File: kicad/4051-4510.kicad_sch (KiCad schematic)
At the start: 10 parts, among them U19 CD4051B, U20 4510

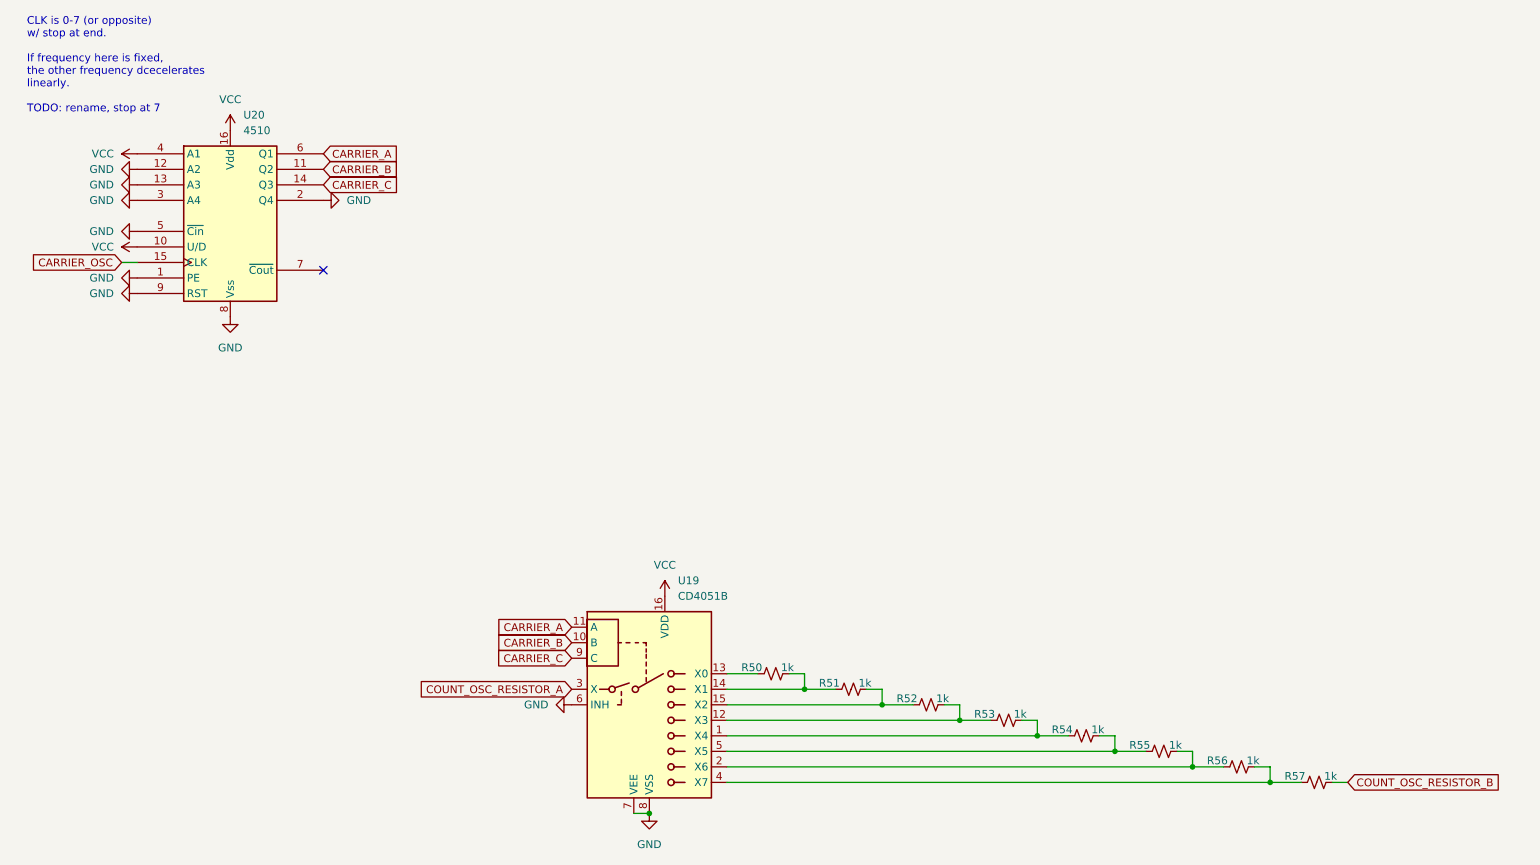
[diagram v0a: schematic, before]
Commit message: CONTINUE
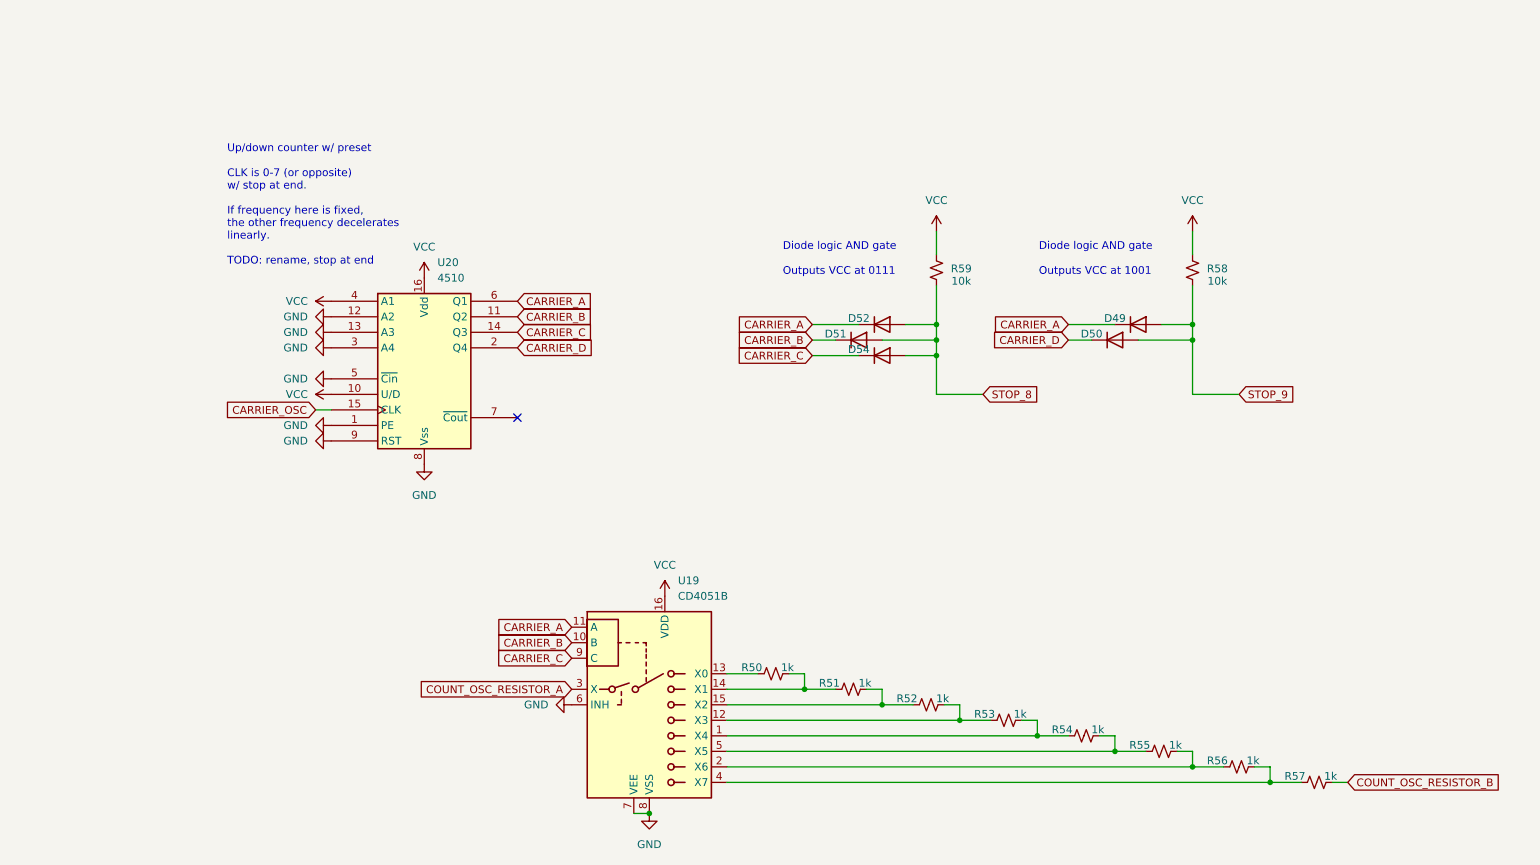
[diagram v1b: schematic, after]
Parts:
- added D49, D50, D51, D52, D54: 1N4148WT, Diode_SMD:D_SOD-523, symbol Diode:1N4148WT
- added R58, R59: 10k, symbol Device:R_Small_US
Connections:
- net CARRIER_A: now also D49.1 (K), D52.1 (K)
- net CARRIER_B: now also D51.1 (K)
- net CARRIER_C: now also D54.1 (K)
- net GND: no longer U20.2 (Q4)
- net VCC: now also R58.2, R59.2
- new net CARRIER_D: D50.1 (K), U20.2 (Q4)
- new net STOP_8: D51.2 (A), D52.2 (A), D54.2 (A), R59.1
- new net STOP_9: D49.2 (A), D50.2 (A), R58.1
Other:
- note added: "Diode logic AND gate Outputs VCC at 0111"
- note added: "Diode logic AND gate Outputs VCC at 1001"
- note added: "Up/down counter w/ preset CLK is 0-7 (or opposite) w/ stop at end. If frequency here is fixed, the other frequency decelerates linearly. TODO: rename, stop at end"
- note removed: "CLK is 0-7 (or opposite) w/ stop at end. If frequency here is fixed, the other frequency dcecelerates linearly. TODO: rename, stop at 7"
- moved on the sheet: U20
